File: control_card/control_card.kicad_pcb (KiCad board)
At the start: 2 copper layers, 71.6 x 49.4 mm, 38 parts, among them IC1 TLSR8253F512ET48, J1 Conn_02x04_Counter_Clockwise, U1 Wifi, Y1 Crystal_GND24_Small

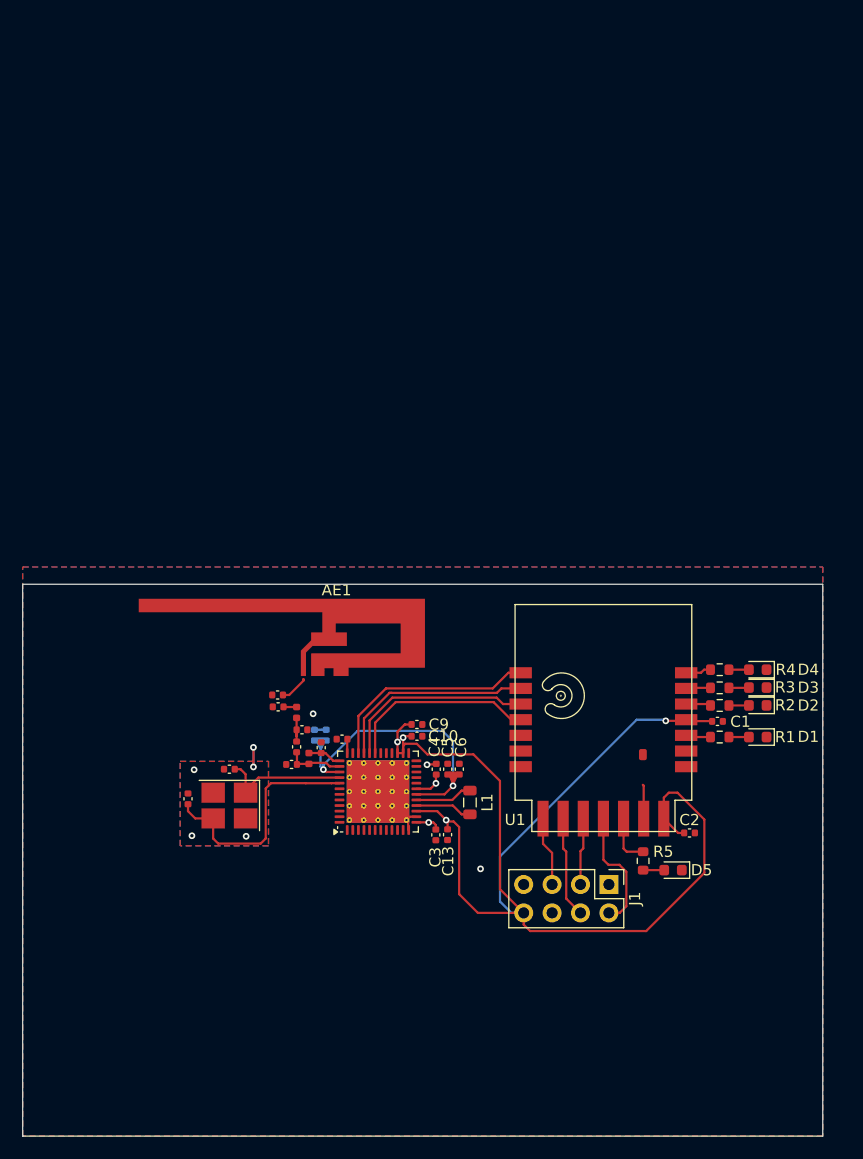
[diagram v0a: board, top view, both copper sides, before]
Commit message: PCB (control_card): Almost Finished
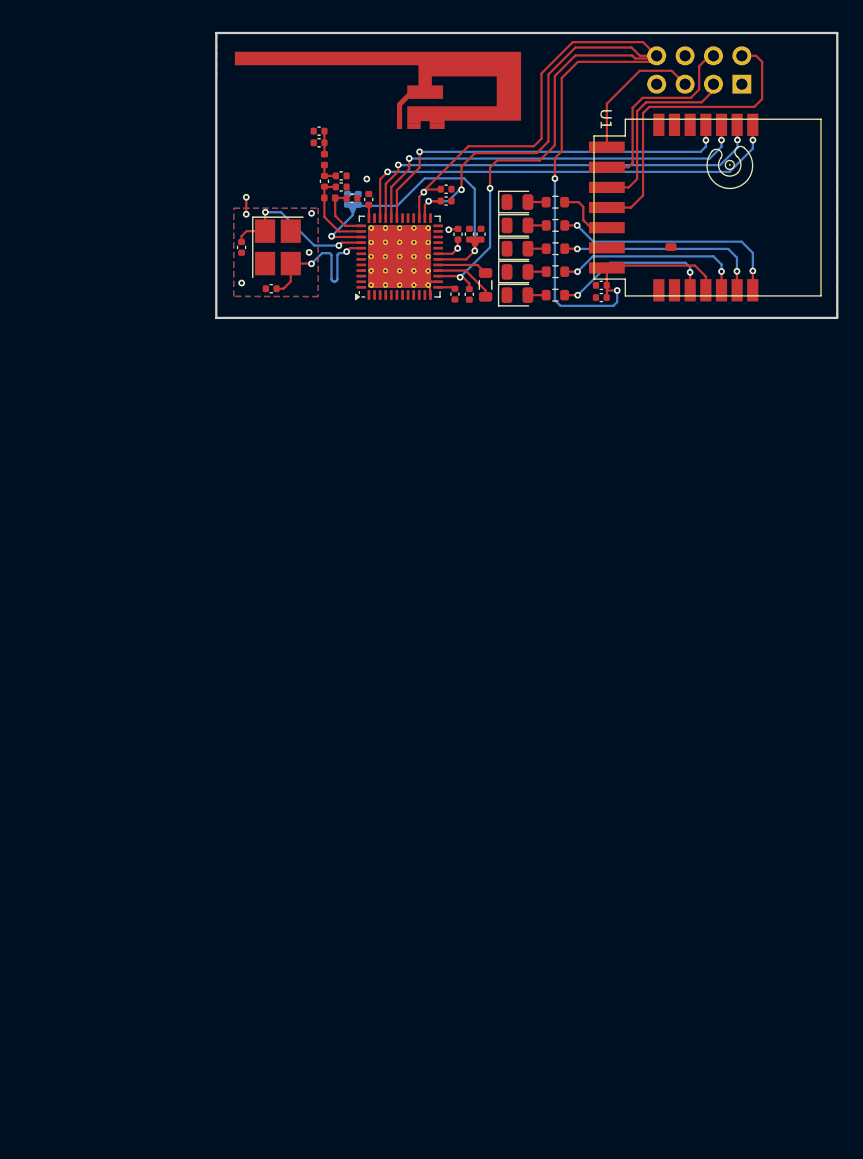
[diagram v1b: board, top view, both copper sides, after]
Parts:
- AE1: value Antenna -> Antenna_Shield
- D1, D2, D3, D4, D5: footprint LED_SMD:LED_0603_1608Metric -> LED_SMD:LED_0805_2012Metric
- J1: moved to B.Cu
- moved J1 72.5 mm to (109.2, 21.6), turned to 90 degrees
- moved D5 61.3 mm to (89.2, 32.1), turned to 0 degrees
- moved R5 59.4 mm to (92.5, 32.1), turned to 180 degrees
- moved C15 51.8 mm to (73.4, 30.8), turned to 0 degrees
- moved U1 51.3 mm to (116.3, 24.7), turned to -90 degrees
- moved C16 50.6 mm to (71.9, 30.3)
- moved C18 50.6 mm to (71.4, 26.8)
- moved C19 50.6 mm to (71.4, 25.8)
- moved D1 50.5 mm to (89.2, 34.2), turned to 0 degrees
- moved L2 50.2 mm to (72.4, 31.8), turned to 0 degrees
- moved Y1 50.1 mm to (67.7, 36.2), turned to -90 degrees
- moved C17 49.7 mm to (73.4, 29.8)
- moved C2 49.6 mm to (96.7, 39.6), turned to 180 degrees
- moved L3 49.5 mm to (71.9, 28.3)
- moved C14 49.2 mm to (74.3, 31.8), turned to 0 degrees
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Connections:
- R1 pad 1: Led_1 -> Led_4
- R2 pad 1: Led_2 -> Led_3
- R3 pad 1: Led_3 -> Led_2
- R4 pad 1: Led_4 -> Led_1
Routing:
- net +3.3V: track 111.3 -> 156.5 mm, vias 4 -> 7
- net In_1: track 19.4 -> 40.1 mm, vias 0 -> 2
- net In_2: track 18.4 -> 38.3 mm, vias 0 -> 2
- net Led_4: track 2.29 -> 21.2 mm, vias 0 -> 2
- net In_3: track 17.5 -> 36.3 mm, vias 0 -> 2
- net In_4: track 17.2 -> 34.5 mm, vias 0 -> 2
- net CT4: track 11.1 -> 27.6 mm
- net Led_3: track 2.20 -> 18.7 mm, vias 0 -> 2
- net Led_2: track 2.23 -> 17.2 mm, vias 0 -> 2
- net Led_1: track 2.24 -> 14.6 mm, vias 0 -> 2
- net CT3: track 5.99 -> 17.2 mm
- net CT2: track 9.07 -> 17.8 mm
- net Clock2: track 21.3 -> 14.7 mm, vias 0 -> 2
- net CT1: track 6.22 -> 12.6 mm
- net GND: track 10.3 -> 5.25 mm, vias 8 -> 7
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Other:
- board size 71.6 x 49.4 mm -> 55.5 x 25.5 mm

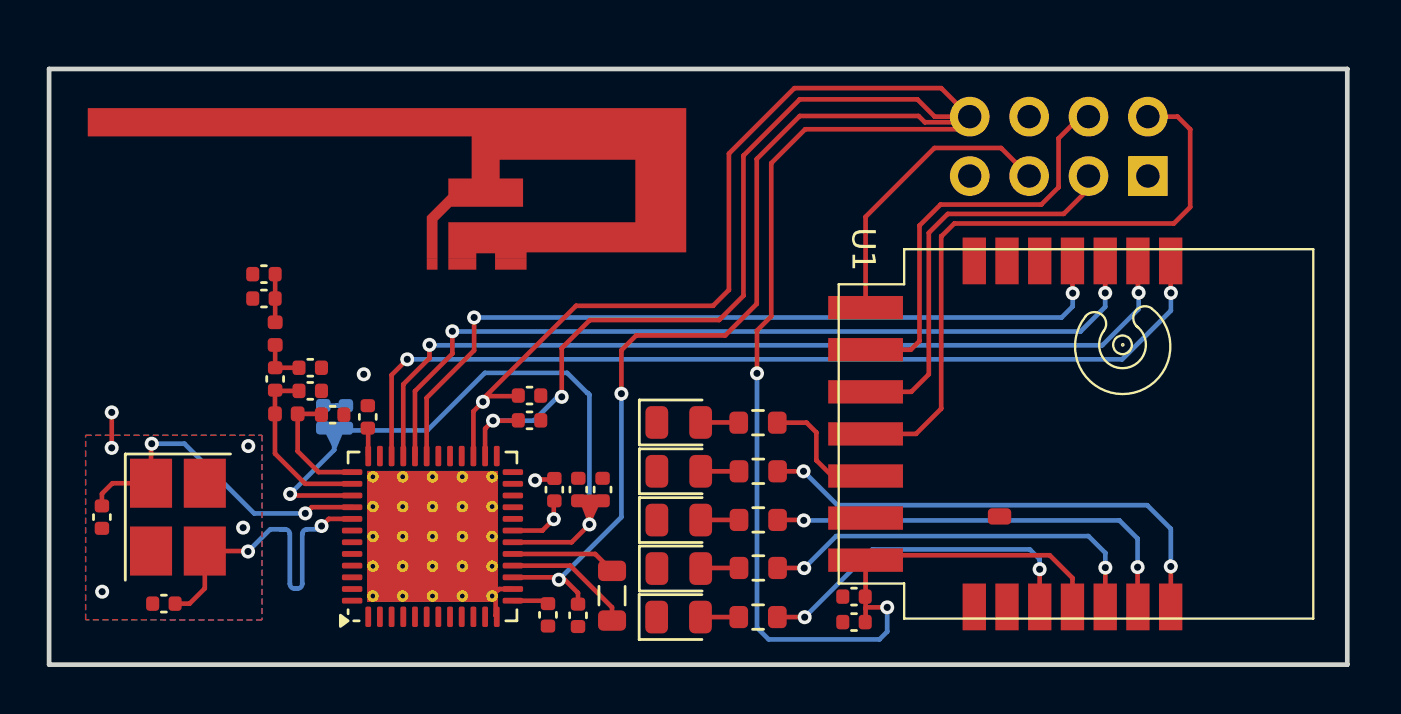
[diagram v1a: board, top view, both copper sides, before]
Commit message: PCB (control_card) : V1 finished
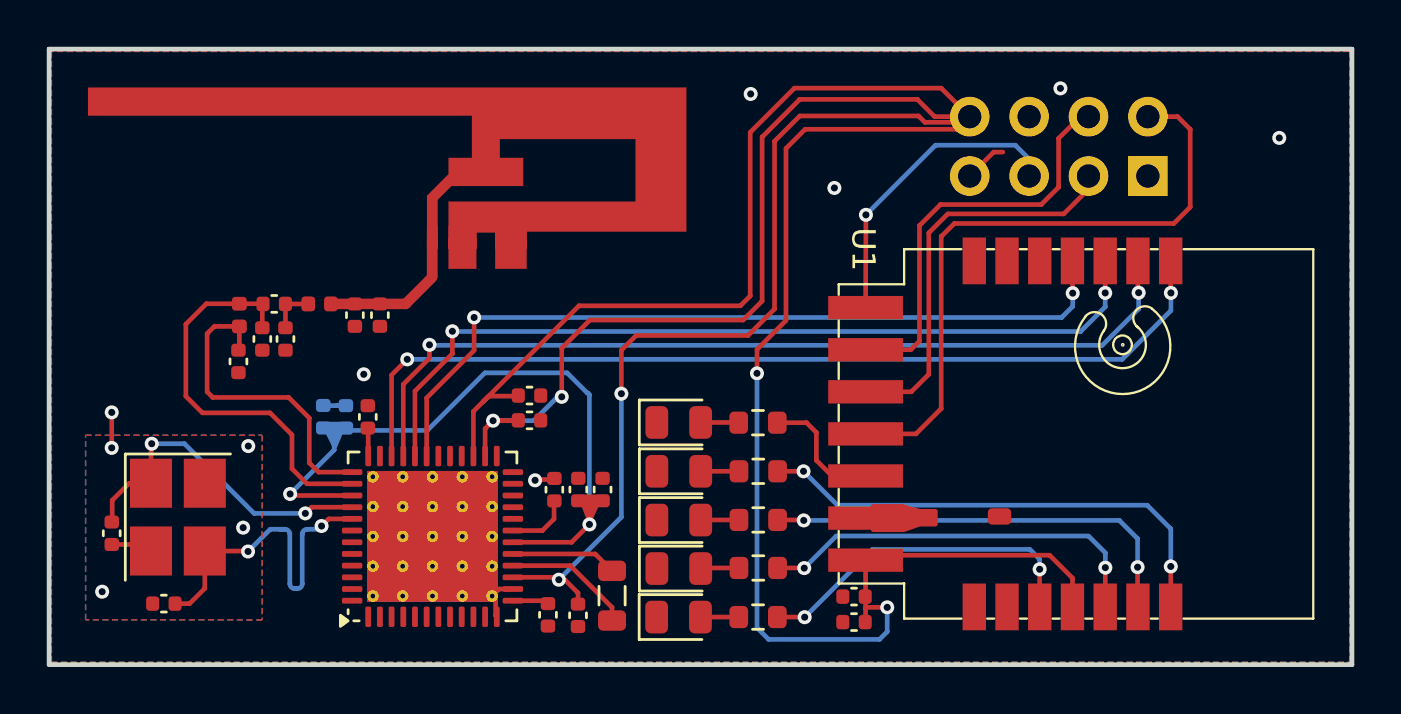
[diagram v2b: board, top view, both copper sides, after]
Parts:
- moved C19 5.26 mm to (76.4, 27.5), turned to -90 degrees
- moved L2 4.68 mm to (70.4, 27.5), turned to -90 degrees
- moved C14 4.63 mm to (70.3, 29.5), turned to -90 degrees
- moved C18 3.95 mm to (75.3, 27.5), turned to -90 degrees
- moved C16 3.21 mm to (71.8, 27.1), turned to 0 degrees
- moved C15 3.02 mm to (71.3, 28.6), turned to -90 degrees
- moved L3 2.29 mm to (73.8, 27.1), turned to 0 degrees
- moved C17 1.62 mm to (72.3, 28.6), turned to -90 degrees
- moved AE1 0.89 mm to (81.6, 23.1)
- moved C11 0.81 mm to (64.9, 36.9)
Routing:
- net GND: track 5.25 -> 29.9 mm, vias 7 -> 11
- net ANT: track 7.72 -> 17.4 mm
- net VANT: track 5.33 -> 13.8 mm
- net Net-(AE1-A): track 2.08 -> 4.83 mm
- net +3.3V: track 156.5 -> 158.3 mm, vias 7 -> 6
- net CT1: track 12.6 -> 13.2 mm, vias 0 -> 1
- net VDD_F: track 2.66 -> 2.74 mm, vias 1 -> 0
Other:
- board size 55.5 x 25.5 mm -> 55.7 x 26.3 mm
